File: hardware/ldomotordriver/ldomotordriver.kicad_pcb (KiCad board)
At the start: 2 copper layers, 17.5 x 27.5 mm, 15 parts, among them U1 AMS1117-3.3, U2 DRV8870DDA

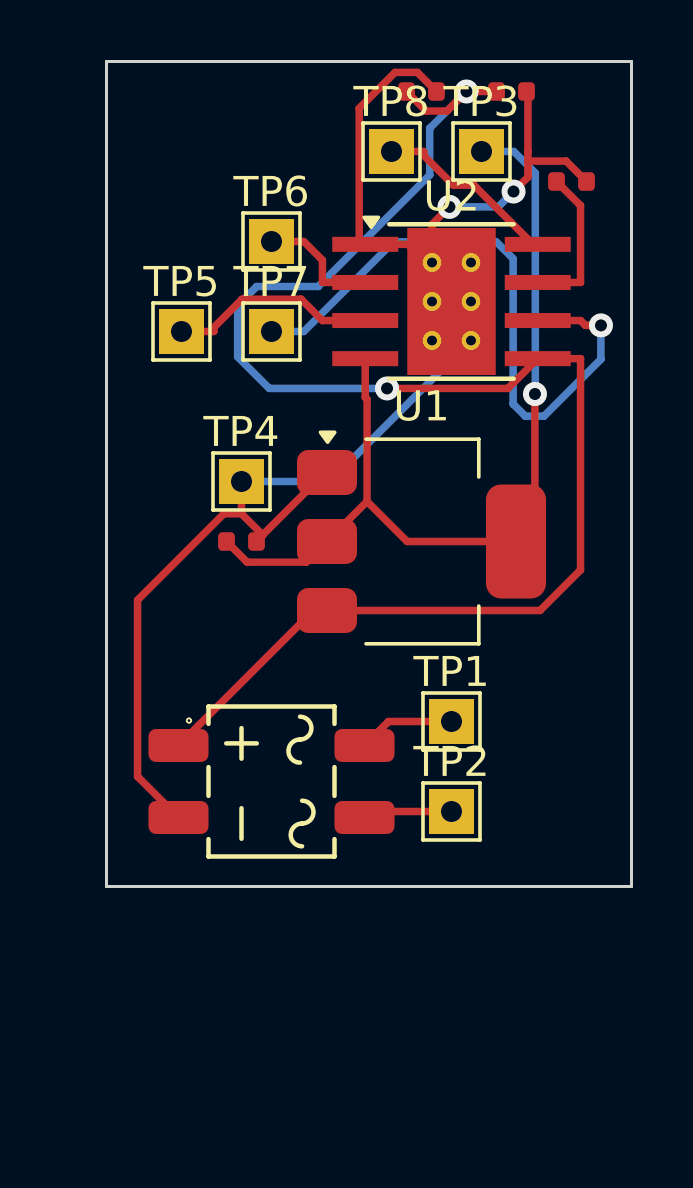
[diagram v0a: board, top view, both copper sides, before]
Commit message: gnd zones
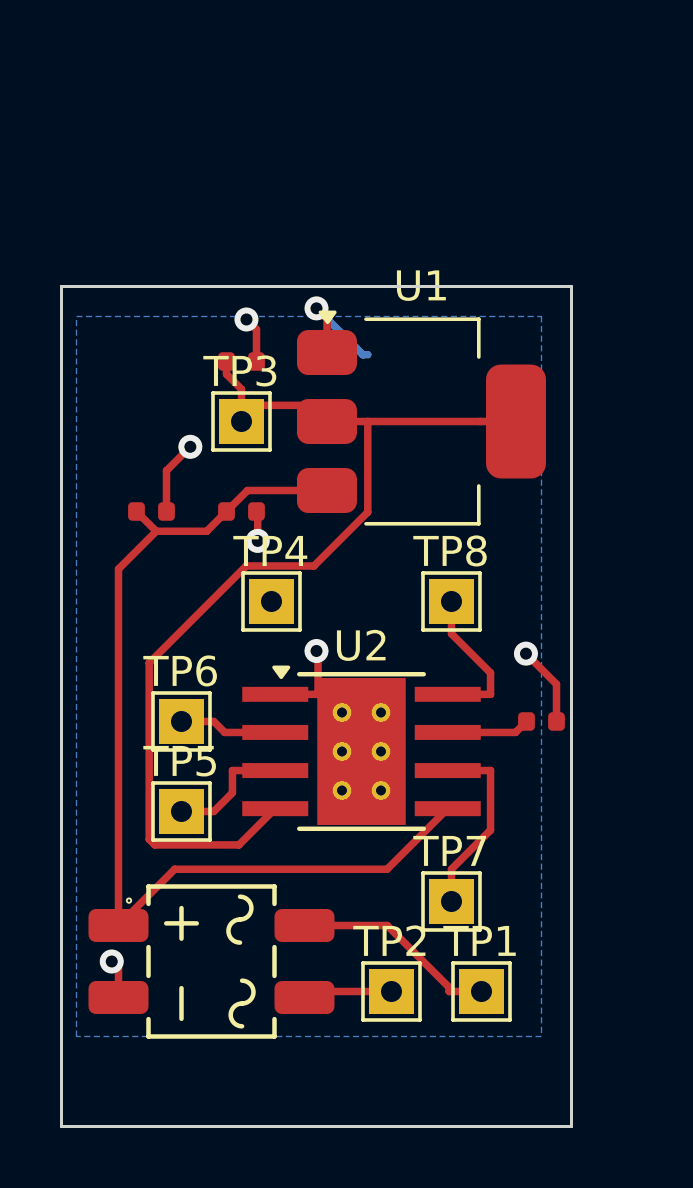
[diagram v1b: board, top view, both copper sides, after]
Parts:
- R1: value 0.2 -> C270629
- moved TP7 19.9 mm to (95.0, 60.0)
- moved R1 18.0 mm to (98.0, 54.0)
- moved C1 16.6 mm to (85.0, 47.0)
- moved C3 16.6 mm to (88.0, 47.0)
- moved TP6 16.3 mm to (86.0, 54.0)
- moved TP5 16.0 mm to (86.0, 57.0)
- moved U2 15.3 mm to (92.0, 55.0)
- moved TP8 15.1 mm to (95.0, 50.0)
- moved TP3 12.0 mm to (88.0, 44.0)
- moved TP1 9.06 mm to (96.0, 63.0)
- moved DB1 6.32 mm to (87.0, 62.0)
- moved TP2 6.32 mm to (93.0, 63.0)
- moved C2 6.00 mm to (88.0, 42.0)
- moved TP4 4.12 mm to (89.0, 50.0)
- moved U1 4.00 mm to (94.0, 44.0)
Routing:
- net GND: track 55.7 -> 16.8 mm, vias 2 -> 7
- net Net-(DB1-+): track 52.4 -> 33.4 mm, vias 2 -> 0
- net Net-(U2-OUT1): track 23.1 -> 6.33 mm, vias 1 -> 0
- net Net-(U1-VO): track 30.8 -> 34.6 mm, vias 1 -> 0
- net Net-(DB1-AC-Pad4): track 3.23 -> 6.89 mm
- net Net-(U2-IN1): track 6.94 -> 4.13 mm
- net Net-(U2-ISEN): track 5.12 -> 2.78 mm
- net Net-(U2-OUT2): track 6.24 -> 5.06 mm
- net Net-(U2-IN2): track 4.13 -> 3.28 mm
- added copper zone on B.Cu, net GND
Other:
- board size 17.5 x 27.5 mm -> 17 x 28 mm
